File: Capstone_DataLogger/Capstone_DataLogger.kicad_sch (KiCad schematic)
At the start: 1 part

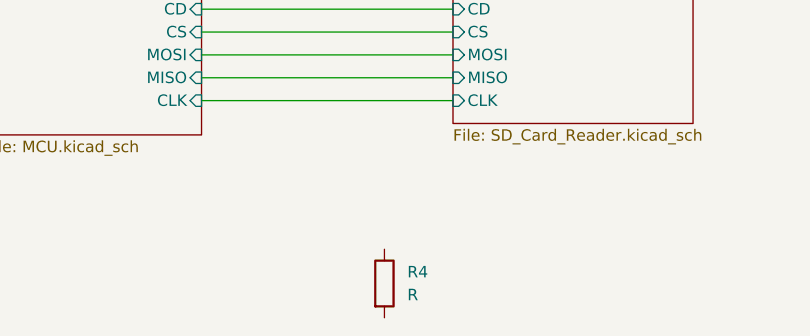
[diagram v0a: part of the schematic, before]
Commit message: basic changes
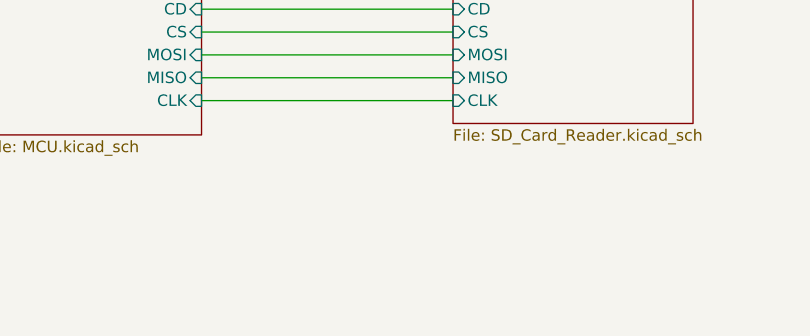
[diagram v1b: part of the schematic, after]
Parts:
- removed R4: R, symbol Device:R
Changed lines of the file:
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@@
-		)
-	)
-	(symbol
-		(lib_id "Device:R")
-		(at 170.18 129.54 0)
-		(unit 1)
-		(exclude_from_sim no)
-		(in_bom yes)
-		(on_board yes)
-		(dnp no)
-		(fields_autoplaced yes)
-		(property "Reference" "R4"
-			(at 172.72 128.2699 0)
-			(effects
-				(font
-					(size 1.27 1.27)
-				)
-				(justify left)
-			)
-		)
-		(property "Value" "R"
-			(at 172.72 130.8099 0)
-			(effects
-				(font
-					(size 1.27 1.27)
-				)
-				(justify left)
-			)
-		)
-		(property "Footprint" ""
-			(at 168.402 129.54 90)
-			(effects
-				(font
-					(size 1.27 1.27)
-				)
-				(hide yes)
-			)
-		)
-		(property "Datasheet" "~"
-			(at 170.18 129.54 0)
-			(effects
-				(font
-					(size 1.27 1.27)
-				)
-				(hide yes)
-			)
-		)
-		(property "Description" "Resistor"
-			(at 170.18 129.54 0)
-			(effects
-				(font
-					(size 1.27 1.27)
-				)
-				(hide yes)
-			)
-		)
-		(pin "2"
-		)
-		(pin "1"
-		)
-		(instances
-			(project ""
-				(path "/3b56a84b-c06c-4c22-a01a-903db63bf091"
-					(reference "R4")
-					(unit 1)
-				)
-			)
 		)
 	)
